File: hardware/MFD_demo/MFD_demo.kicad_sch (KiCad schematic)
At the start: 36 parts, among them J1 Pins_Ard, J2 POWER, Q1 IRF740, Q2 IRF740, Q3 IRF740, Q4 IRF740, Q5 IRF740, Q6 IRF740

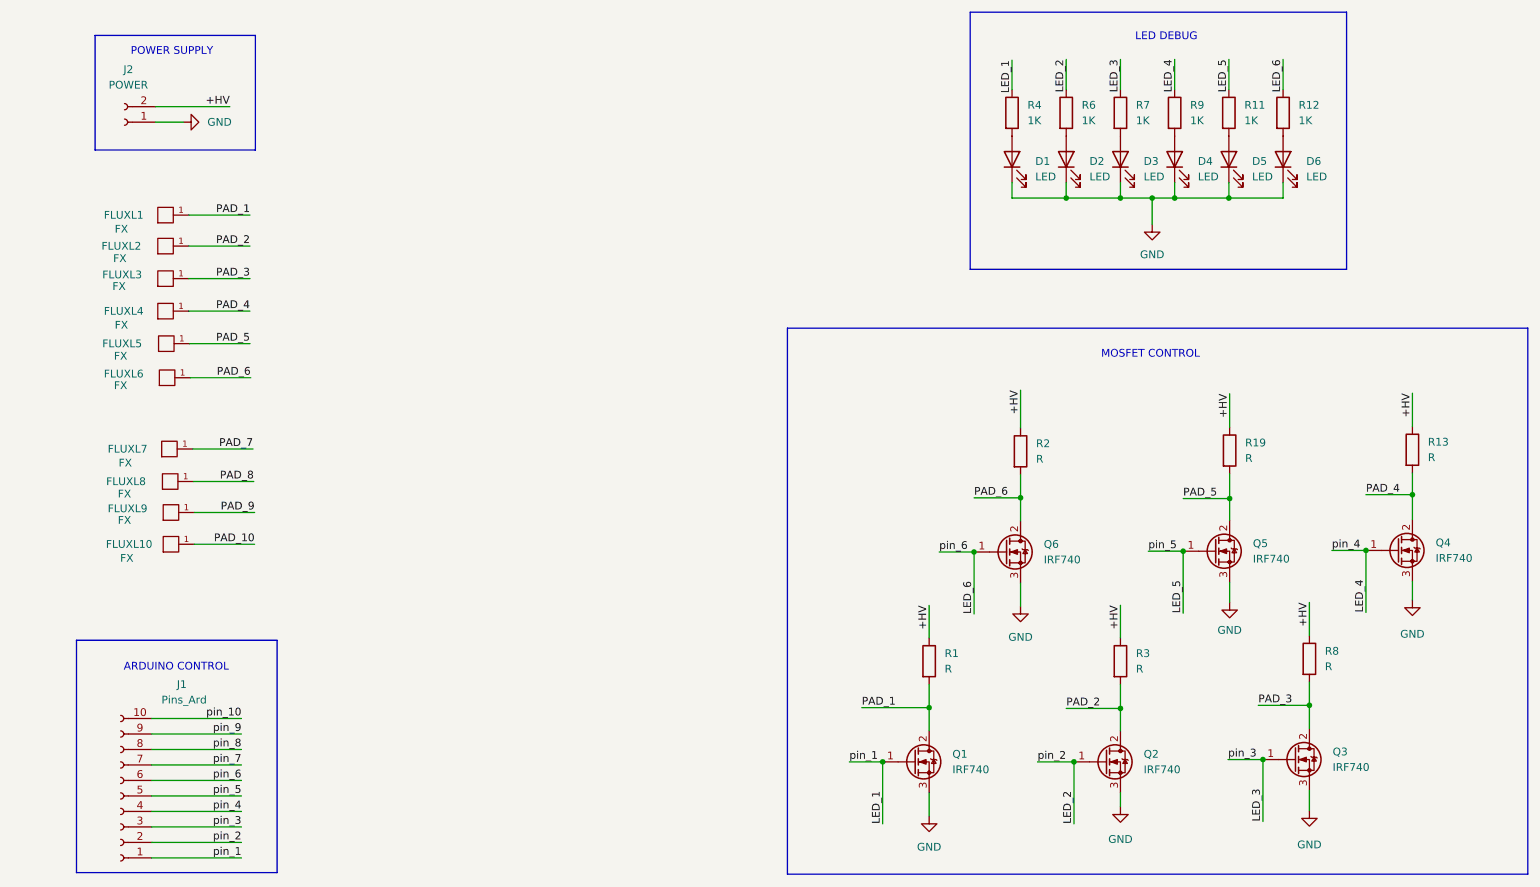
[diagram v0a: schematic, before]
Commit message: Update PCB layout version 01
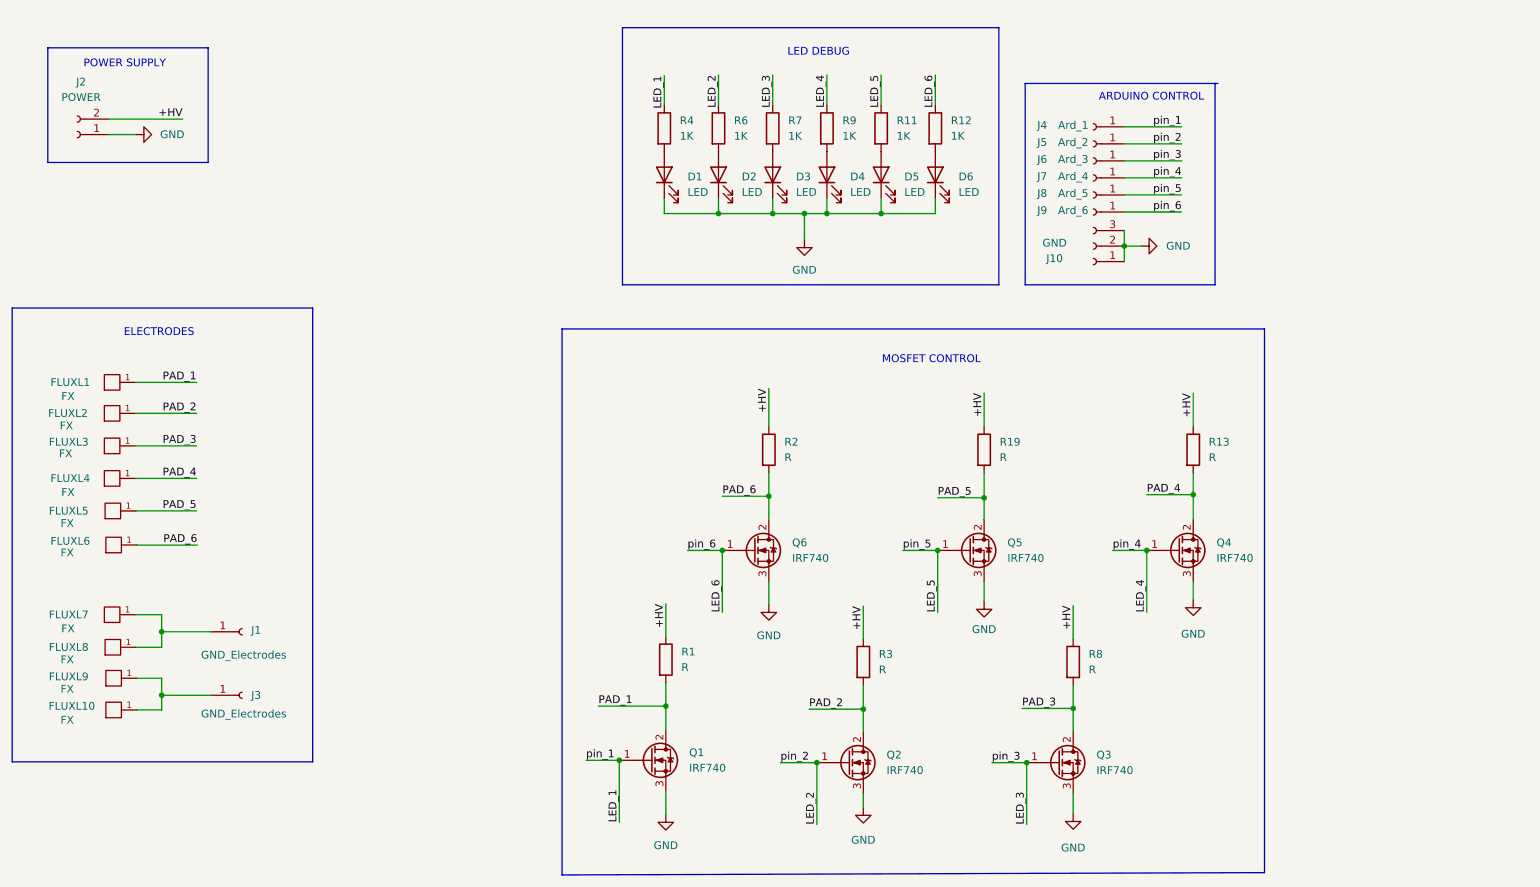
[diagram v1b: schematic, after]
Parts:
- removed J1: Pins_Ard, Connector_PinHeader_2.54mm:PinHeader_1x10_P2.54mm_Vertical, symbol Connector:Conn_01x10_Female
- added J1, J3: GND_Electrodes, Connector_PinSocket_2.54mm:PinSocket_1x01_P2.54mm_Vertical, symbol Connector:Conn_01x01_Female
- added J10: GND, Connector_PinSocket_2.54mm:PinSocket_1x03_P2.54mm_Vertical, symbol Connector:Conn_01x03_Female
- added J4: Ard_1, Connector_PinSocket_2.54mm:PinSocket_1x01_P2.54mm_Vertical, symbol Connector:Conn_01x01_Female
- added J5: Ard_2, Connector_PinSocket_2.54mm:PinSocket_1x01_P2.54mm_Vertical, symbol Connector:Conn_01x01_Female
- added J6: Ard_3, Connector_PinSocket_2.54mm:PinSocket_1x01_P2.54mm_Vertical, symbol Connector:Conn_01x01_Female
- added J7: Ard_4, Connector_PinSocket_2.54mm:PinSocket_1x01_P2.54mm_Vertical, symbol Connector:Conn_01x01_Female
- added J8: Ard_5, Connector_PinSocket_2.54mm:PinSocket_1x01_P2.54mm_Vertical, symbol Connector:Conn_01x01_Female
- added J9: Ard_6, Connector_PinSocket_2.54mm:PinSocket_1x01_P2.54mm_Vertical, symbol Connector:Conn_01x01_Female
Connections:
- net PAD_8 is gone; now on an unnamed net: FLUXL8.1
- net PAD_9 is gone; now on an unnamed net: FLUXL9.1
- net GND: now also J10.1 (Pin_1), J10.2 (Pin_2), J10.3 (Pin_3)
- net LED_1: now also J4.1 (Pin_1)
- net LED_2: now also J5.1 (Pin_1)
- net LED_3: now also J6.1 (Pin_1)
- net LED_4: now also J7.1 (Pin_1)
- net LED_5: now also J8.1 (Pin_1)
- net LED_6: now also J9.1 (Pin_1)
- net PAD_10: no longer names the net of FLUXL10.1
- net PAD_10: now also J3.1 (Pin_1)
- net PAD_7: no longer names the net of FLUXL7.1
- net PAD_7: now also J1.1 (Pin_1)
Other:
- note added: "ELECTRODES"
- moved on the sheet: D1, D2, D3, D4, D5, D6, FLUXL1, FLUXL10, FLUXL2, FLUXL3, FLUXL4, FLUXL5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

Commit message: Update PCB layout
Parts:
- R1, R11, R12, R13, R19, R2, R3, R4, R6, R7, R8, R9: footprint Resistor_THT:R_Axial_DIN0204_L3.6mm_D1.6mm_P5.08mm_Horizontal -> Resistor_THT:R_Axial_DIN0207_L6.3mm_D2.5mm_P10.16mm_Horizontal
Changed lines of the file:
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@@
       (effects (font (size 1.27 1.27)) (justify left))
     )
-    (property "Footprint" "Resistor_THT:R_Axial_DIN0204_L3.6mm_D1.6mm_P5.08mm_Horizontal" (id 2) (at 169.545 128.905 90)
+    (property "Footprint" "Resistor_THT:R_Axial_DIN0207_L6.3mm_D2.5mm_P10.16mm_Horizontal" (id 2) (at 169.545 128.905 90)
       (effects (font (size 1.27 1.27)) hide)
     )
@@
       (effects (font (size 1.27 1.27)) (justify left))
     )
-    (property "Footprint" "Resistor_THT:R_Axial_DIN0204_L3.6mm_D1.6mm_P5.08mm_Horizontal" (id 2) (at 154.051 94.107 90)
+    (property "Footprint" "Resistor_THT:R_Axial_DIN0207_L6.3mm_D2.5mm_P10.16mm_Horizontal" (id 2) (at 154.051 94.107 90)
       (effects (font (size 1.27 1.27)) hide)
     )
@@
       (effects (font (size 1.27 1.27)) (justify left))
     )
-    (property "Footprint" "Resistor_THT:R_Axial_DIN0204_L3.6mm_D1.6mm_P5.08mm_Horizontal" (id 2) (at 203.962 128.905 90)
+    (property "Footprint" "Resistor_THT:R_Axial_DIN0207_L6.3mm_D2.5mm_P10.16mm_Horizontal" (id 2) (at 203.962 128.905 90)
       (effects (font (size 1.27 1.27)) hide)
     )
@@
       (effects (font (size 1.27 1.27)) (justify left))
     )
-    (property "Footprint" "Resistor_THT:R_Axial_DIN0204_L3.6mm_D1.6mm_P5.08mm_Horizontal" (id 2) (at 189.357 94.107 90)
+    (property "Footprint" "Resistor_THT:R_Axial_DIN0207_L6.3mm_D2.5mm_P10.16mm_Horizontal" (id 2) (at 189.357 94.107 90)
       (effects (font (size 1.27 1.27)) hide)
     )
@@
       (effects (font (size 1.27 1.27)) (justify left))
     )
-    (property "Footprint" "Resistor_THT:R_Axial_DIN0204_L3.6mm_D1.6mm_P5.08mm_Horizontal" (id 2) (at 181.356 41.402 90)
+    (property "Footprint" "Resistor_THT:R_Axial_DIN0207_L6.3mm_D2.5mm_P10.16mm_Horizontal" (id 2) (at 181.356 41.402 90)
       (effects (font (size 1.27 1.27)) hide)
     )
@@
       (effects (font (size 1.27 1.27)) (justify left))
     )
-    (property "Footprint" "Resistor_THT:R_Axial_DIN0204_L3.6mm_D1.6mm_P5.08mm_Horizontal" (id 2) (at 154.686 41.402 90)
+    (property "Footprint" "Resistor_THT:R_Axial_DIN0207_L6.3mm_D2.5mm_P10.16mm_Horizontal" (id 2) (at 154.686 41.402 90)
       (effects (font (size 1.27 1.27)) hide)
     )
@@
       (effects (font (size 1.27 1.27)) (justify left))
     )
-    (property "Footprint" "Resistor_THT:R_Axial_DIN0204_L3.6mm_D1.6mm_P5.08mm_Horizontal" (id 2) (at 223.647 94.107 90)
+    (property "Footprint" "Resistor_THT:R_Axial_DIN0207_L6.3mm_D2.5mm_P10.16mm_Horizontal" (id 2) (at 223.647 94.107 90)
       (effects (font (size 1.27 1.27)) hide)
     )
@@
       (effects (font (size 1.27 1.27)) (justify left))
     )
-    (property "Footprint" "Resistor_THT:R_Axial_DIN0204_L3.6mm_D1.6mm_P5.08mm_Horizontal" (id 2) (at 172.466 41.402 90)
+    (property "Footprint" "Resistor_THT:R_Axial_DIN0207_L6.3mm_D2.5mm_P10.16mm_Horizontal" (id 2) (at 172.466 41.402 90)
       (effects (font (size 1.27 1.27)) hide)
     )
@@
       (effects (font (size 1.27 1.27)) (justify left))
     )
-    (property "Footprint" "Resistor_THT:R_Axial_DIN0204_L3.6mm_D1.6mm_P5.08mm_Horizontal" (id 2) (at 136.906 41.402 90)
+    (property "Footprint" "Resistor_THT:R_Axial_DIN0207_L6.3mm_D2.5mm_P10.16mm_Horizontal" (id 2) (at 136.906 41.402 90)
       (effects (font (size 1.27 1.27)) hide)
     )
@@
       (effects (font (size 1.27 1.27)) (justify left))
     )
-    (property "Footprint" "Resistor_THT:R_Axial_DIN0204_L3.6mm_D1.6mm_P5.08mm_Horizontal" (id 2) (at 137.16 128.524 90)
+    (property "Footprint" "Resistor_THT:R_Axial_DIN0207_L6.3mm_D2.5mm_P10.16mm_Horizontal" (id 2) (at 137.16 128.524 90)
       (effects (font (size 1.27 1.27)) hide)
     )
@@
       (effects (font (size 1.27 1.27)) (justify left))
     )
-    (property "Footprint" "Resistor_THT:R_Axial_DIN0204_L3.6mm_D1.6mm_P5.08mm_Horizontal" (id 2) (at 145.796 41.402 90)
+    (property "Footprint" "Resistor_THT:R_Axial_DIN0207_L6.3mm_D2.5mm_P10.16mm_Horizontal" (id 2) (at 145.796 41.402 90)
       (effects (font (size 1.27 1.27)) hide)
     )
@@
       (effects (font (size 1.27 1.27)) (justify left))
     )
-    (property "Footprint" "Resistor_THT:R_Axial_DIN0204_L3.6mm_D1.6mm_P5.08mm_Horizontal" (id 2) (at 163.576 41.402 90)
+    (property "Footprint" "Resistor_THT:R_Axial_DIN0207_L6.3mm_D2.5mm_P10.16mm_Horizontal" (id 2) (at 163.576 41.402 90)
       (effects (font (size 1.27 1.27)) hide)
     )
@@
     )
     (path "/be0a93d4-c7fe-4417-b63d-cae7dd23acfb"
-      (reference "R1") (unit 1) (value "R") (footprint "Resistor_THT:R_Axial_DIN0204_L3.6mm_D1.6mm_P5.08mm_Horizontal")
+      (reference "R1") (unit 1) (value "R") (footprint "Resistor_THT:R_Axial_DIN0207_L6.3mm_D2.5mm_P10.16mm_Horizontal")
     )
     (path "/27ad1b76-a7b6-4284-b8ed-9188bd611cd9"
-      (reference "R2") (unit 1) (value "R") (footprint "Resistor_THT:R_Axial_DIN0204_L3.6mm_D1.6mm_P5.08mm_Horizontal")
+      (reference "R2") (unit 1) (value "R") (footprint "Resistor_THT:R_Axial_DIN0207_L6.3mm_D2.5mm_P10.16mm_Horizontal")
     )
     (path "/05d574de-583c-416b-a316-989f3cd535f3"
-      (reference "R3") (unit 1) (value "R") (footprint "Resistor_THT:R_Axial_DIN0204_L3.6mm_D1.6mm_P5.08mm_Horizontal")
+      (reference "R3") (unit 1) (value "R") (footprint "Resistor_THT:R_Axial_DIN0207_L6.3mm_D2.5mm_P10.16mm_Horizontal")
     )
     (path "/b710cd78-0899-47ec-87c6-6995f4acff0d"
-      (reference "R4") (unit 1) (value "1K") (footprint "Resistor_THT:R_Axial_DIN0204_L3.6mm_D1.6mm_P5.08mm_Horizontal")
+      (reference "R4") (unit 1) (value "1K") (footprint "Resistor_THT:R_Axial_DIN0207_L6.3mm_D2.5mm_P10.16mm_Horizontal")
     )
     (path "/e09b8ead-9636-4a68-a80a-e4f72d0a1616"
-      (reference "R6") (unit 1) (value "1K") (footprint "Resistor_THT:R_Axial_DIN0204_L3.6mm_D1.6mm_P5.08mm_Horizontal")
+      (reference "R6") (unit 1) (value "1K") (footprint "Resistor_THT:R_Axial_DIN0207_L6.3mm_D2.5mm_P10.16mm_Horizontal")
     )
     (path "/8f5749bc-b397-4181-990f-91932b53985e"
-      (reference "R7") (unit 1) (value "1K") (footprint "Resistor_THT:R_Axial_DIN0204_L3.6mm_D1.6mm_P5.08mm_Horizontal")
+      (reference "R7") (unit 1) (value "1K") (footprint "Resistor_THT:R_Axial_DIN0207_L6.3mm_D2.5mm_P10.16mm_Horizontal")
     )
     (path "/45570490-597d-42e6-ab7e-3269a77d63b4"
-      (reference "R8") (unit 1) (value "R") (footprint "Resistor_THT:R_Axial_DIN0204_L3.6mm_D1.6mm_P5.08mm_Horizontal")
+      (reference "R8") (unit 1) (value "R") (footprint "Resistor_THT:R_Axial_DIN0207_L6.3mm_D2.5mm_P10.16mm_Horizontal")
     )
     (path "/e3976c00-518b-4fdf-bdaf-5cbde63a2a9e"
-      (reference "R9") (unit 1) (value "1K") (footprint "Resistor_THT:R_Axial_DIN0204_L3.6mm_D1.6mm_P5.08mm_Horizontal")
+      (reference "R9") (unit 1) (value "1K") (footprint "Resistor_THT:R_Axial_DIN0207_L6.3mm_D2.5mm_P10.16mm_Horizontal")
     )
     (path "/aac22eac-a078-45d9-8bc1-9712e010cf3f"
-      (reference "R11") (unit 1) (value "1K") (footprint "Resistor_THT:R_Axial_DIN0204_L3.6mm_D1.6mm_P5.08mm_Horizontal")
+      (reference "R11") (unit 1) (value "1K") (footprint "Resistor_THT:R_Axial_DIN0207_L6.3mm_D2.5mm_P10.16mm_Horizontal")
     )
     (path "/76c9ee3e-8eff-43c3-8c23-922c0f01789b"
-      (reference "R12") (unit 1) (value "1K") (footprint "Resistor_THT:R_Axial_DIN0204_L3.6mm_D1.6mm_P5.08mm_Horizontal")
+      (reference "R12") (unit 1) (value "1K") (footprint "Resistor_THT:R_Axial_DIN0207_L6.3mm_D2.5mm_P10.16mm_Horizontal")
     )
     (path "/a00fc1c5-f91b-4fd1-a923-7db550af0d65"
-      (reference "R13") (unit 1) (value "R") (footprint "Resistor_THT:R_Axial_DIN0204_L3.6mm_D1.6mm_P5.08mm_Horizontal")
+      (reference "R13") (unit 1) (value "R") (footprint "Resistor_THT:R_Axial_DIN0207_L6.3mm_D2.5mm_P10.16mm_Horizontal")
     )
     (path "/6f29a0e0-685e-4409-9450-c55658860f84"
-      (reference "R19") (unit 1) (value "R") (footprint "Resistor_THT:R_Axial_DIN0204_L3.6mm_D1.6mm_P5.08mm_Horizontal")
-    )
-  )
+      (reference "R19") (unit 1) (value "R") (footprint "Resistor_THT:R_Axial_DIN0207_L6.3mm_D2.5mm_P10.16mm_Horizontal")
+    )
+  )
